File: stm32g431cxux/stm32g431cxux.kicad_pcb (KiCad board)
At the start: 2 copper layers, 17.8 x 31.8 mm, 20 parts, among them J1 USB2.0_C_v3, J2 ProMicro-LeftPin-NoGND, J3 ProMicro-RightPin, SW1 SW_Push, U1 AMS1117-3.3, U2 STM32G431CBUx

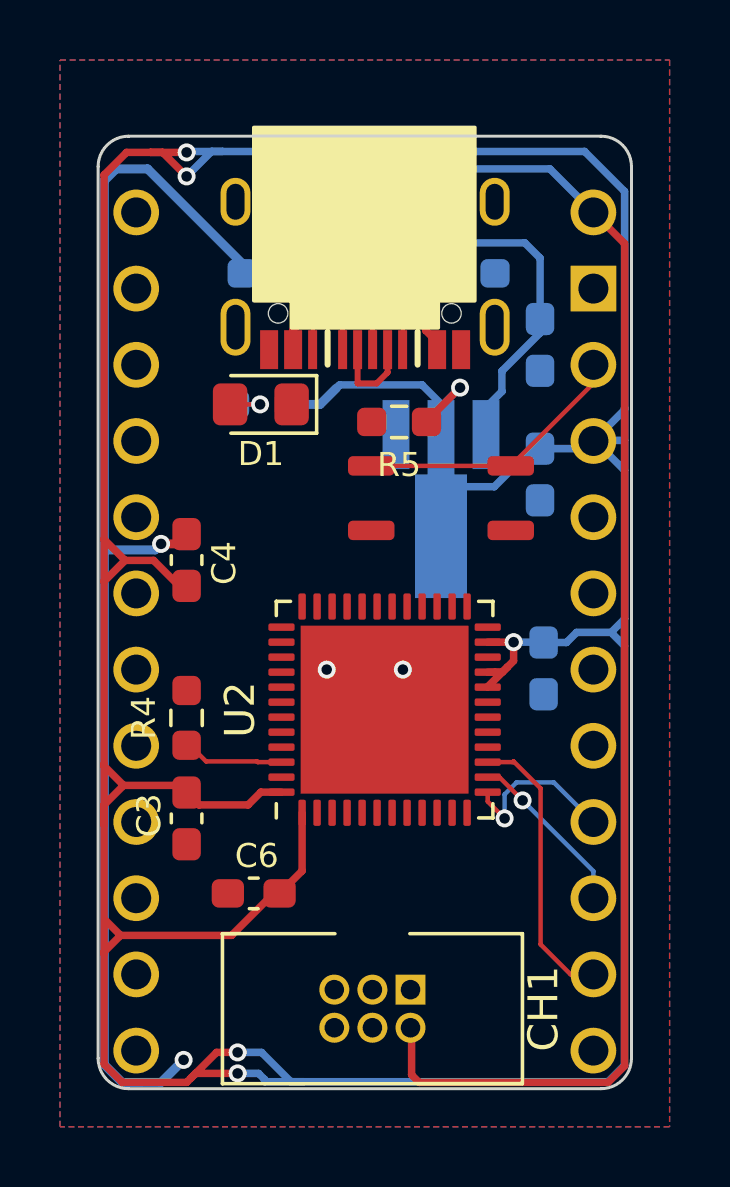
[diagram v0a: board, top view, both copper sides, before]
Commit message: after free routing
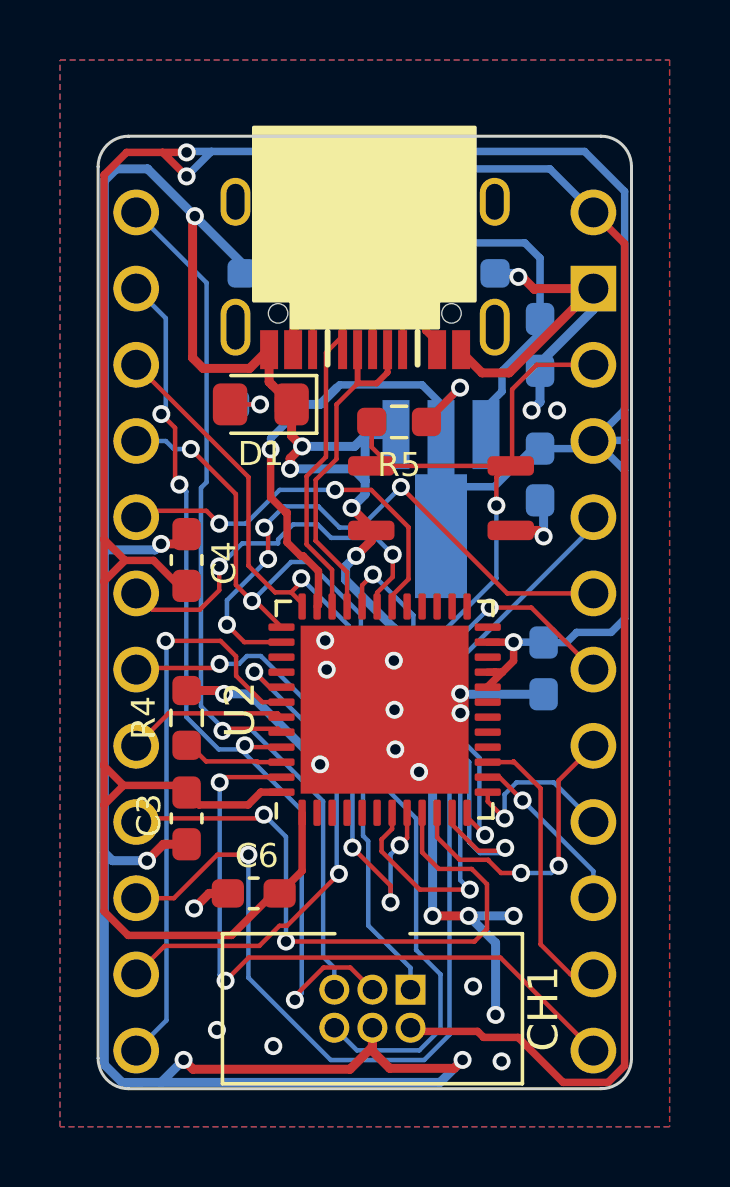
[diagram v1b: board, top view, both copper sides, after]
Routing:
- net GND: track 42.0 -> 139.0 mm, vias 4 -> 32
- net +3V3: track 156.2 -> 116.7 mm, vias 6 -> 5
- net /7: track 0.00 -> 34.2 mm, vias 0 -> 2
- net /SWCLK: track 0.00 -> 33.1 mm, vias 0 -> 2
- net /0/UART_RX: track 0.00 -> 31.5 mm, vias 0 -> 4
- net /1/UART_TX: track 0.00 -> 31.4 mm, vias 0 -> 1
- net /SWDIO: track 0.00 -> 26.5 mm, vias 0 -> 1
- net /NRST: track 9.16 -> 32.8 mm, vias 0 -> 2
- net /10/A10: track 0.00 -> 22.7 mm, vias 0 -> 2
- net /6/A7: track 0.00 -> 21.2 mm, vias 0 -> 2
- net /20/A2: track 0.00 -> 19.5 mm, vias 0 -> 4
- net /9/A9: track 0.00 -> 19.2 mm, vias 0 -> 1
- net /4/A6: track 0.00 -> 17.6 mm, vias 0 -> 4
- net /19/A1: track 0.00 -> 17.4 mm, vias 0 -> 2
- net /8/A9: track 0.00 -> 17.2 mm, vias 0 -> 2
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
